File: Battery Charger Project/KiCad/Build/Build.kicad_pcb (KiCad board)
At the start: 2 copper layers, 135 x 107 mm, 63 parts, among them J1 726386-2, J10 726386-2, J11 726386-2, J2 726386-2, J3 726386-2, J4 Screw_Terminal_01x02, J5 726386-2, J6 726386-2, J7 726386-2, J8 Screw_Terminal_01x05, J9 726386-2, T1 Transformer_SP_1S, U1 LAUNCHXL-F28379D, U2 LNK6773K-TL, U3 MCS1801GS-25-P, U4 L4941BV

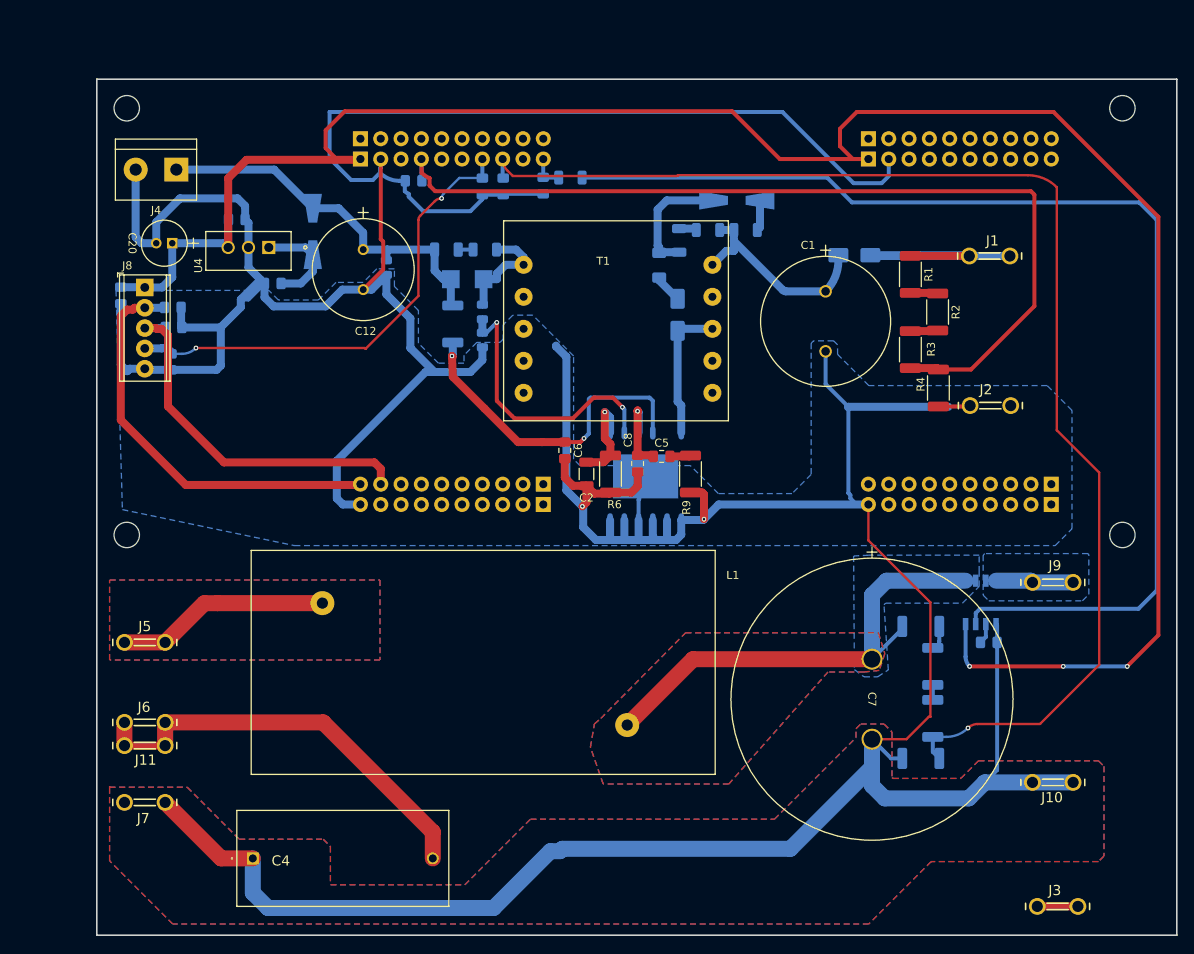
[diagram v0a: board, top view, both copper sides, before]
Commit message: More updates on PCB design
I forgot to push my changes for the last week, but I layed out the components and began routing traces and copper pours.
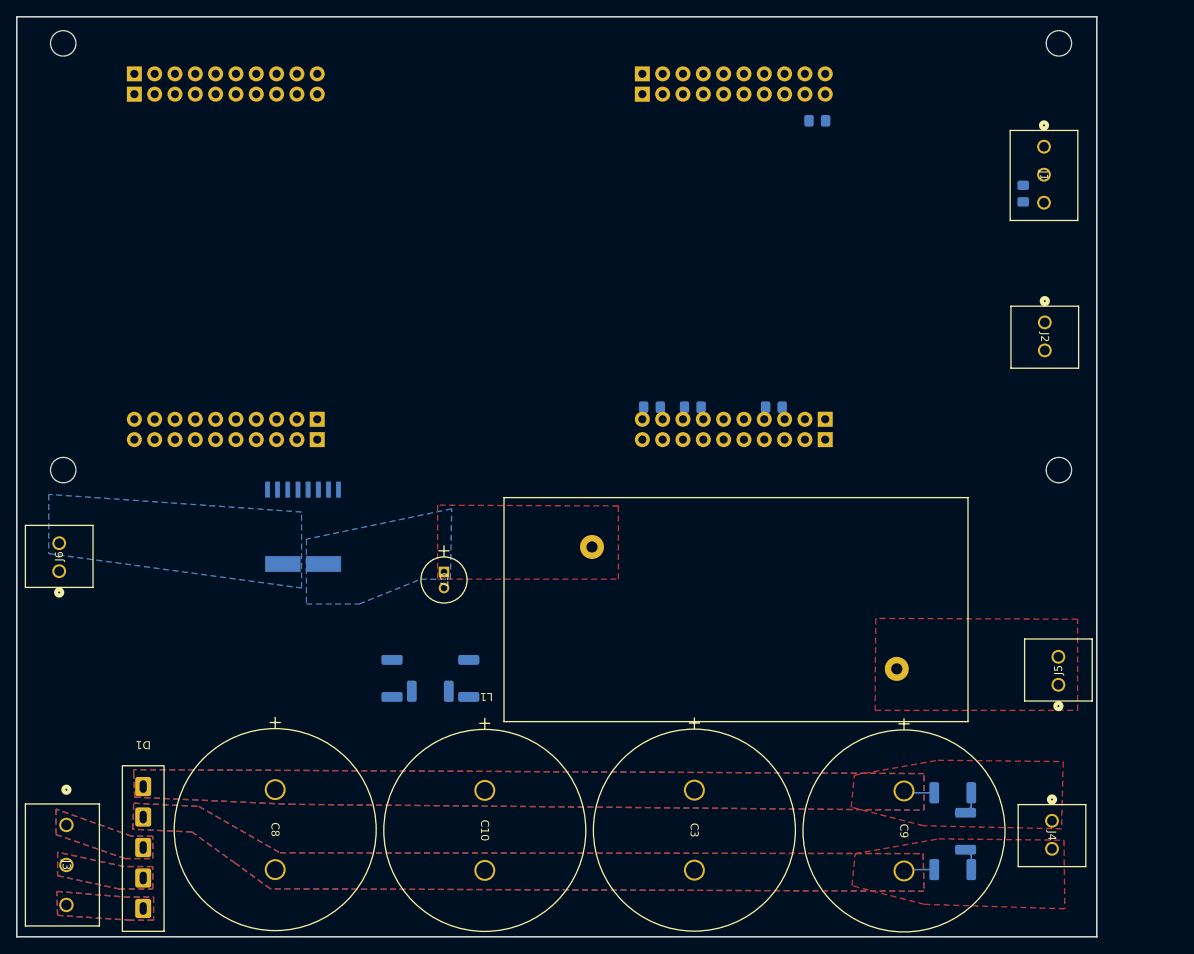
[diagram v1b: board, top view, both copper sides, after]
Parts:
- removed C11, C13, C14, C15, C16, C18, C19: C_Small, Capacitor_SMD:C_0805_2012Metric_Pad1.18x1.45mm_HandSolder
- removed C12: UHE1E102MHD6TO, footprints_C10:CAP_UAQ_12P5X20_NCH
- removed C17, C21: 0.1uF, Capacitor_SMD:C_0805_2012Metric_Pad1.18x1.45mm_HandSolder
- removed C20: ~, footprints_C20:CAP_WCAP-ATG5_05.0X11.0_WRE
- removed D2, D5: D_Zener, Diode_SMD:D_SMA-SMB_Universal_Handsoldering
- removed D3: US1M, Diode_SMD:D_SMA
- removed D4: STPS2H100U, footprints_SCHOTTKYDIODE:SMB_STM
- removed J10, J7, J9: 726386-2, KiCad:726386-2
- removed J11: 726386-2, Library:726386-2
- removed J8: Screw_Terminal_01x05, TerminalBlock_Phoenix:TerminalBlock_Phoenix_MPT-0,5-5-2.54_1x05_P2.54mm_Horizontal
- removed R10, R14, R15, R16, R17, R9: R_Small_US, Resistor_SMD:R_2010_5025Metric
- removed R11, R12, R19: R_Small_US, Resistor_SMD:R_0805_2012Metric
- removed R13: R_Small_US, Resistor_SMD:R_0805_2012Metric_Pad1.20x1.40mm_HandSolder
- removed R18, R20, R7: R_Small_US, Resistor_SMD:R_1206_3216Metric
- removed R8: R_Small_US, Resistor_SMD:R_1206_3216Metric_Pad1.30x1.75mm_HandSolder
- removed T1: Transformer_SP_1S, Library:Transformer_cust_v1
- removed U3: MCS1801GS-25-P, KiCadCS:SOIC127P600X175-8N
- removed U4: L4941BV, L4941BV:TO-220_STM
- C1: value UVR2G220MHD -> C_Small; footprint footprints_C1:CAP_UAQ_16X25_NCH -> Capacitor_SMD:C_0805_2012Metric_Pad1.18x1.45mm_HandSolder; moved to B.Cu
- C10, C3: value C_Small -> ~; footprint Capacitor_SMD:C_1206_3216Metric -> LGW2D561MELA30:CAP_A30_NCH; moved to F.Cu
- C2: footprint Capacitor_SMD:C_1206_3216Metric -> Capacitor_SMD:C_0805_2012Metric_Pad1.18x1.45mm_HandSolder; moved to B.Cu
- C4: value B32673P6225K000 -> C_Small; footprint KiCad_B326:B32673P__26.5_x_12_ -> Capacitor_SMD:C_0805_2012Metric_Pad1.18x1.45mm_HandSolder; moved to B.Cu
- C5, C6: moved to B.Cu
- C7: footprint footprints:CAP_C45_NCH -> EEU-FR1H100:CAP_PAN_5X11_PAN
- C8: value C_Small -> ~; footprint Capacitor_SMD:C_0805_2012Metric_Pad1.18x1.45mm_HandSolder -> LGW2D561MELA30:CAP_A30_NCH
- C9: value C_Small -> ~; footprint Capacitor_SMD:C_0805_2012Metric_Pad1.18x1.45mm_HandSolder -> LGW2D561MELA30:CAP_A30_NCH; moved to F.Cu
- D1: value US1M -> DNA40U2200GU; footprint Diode_SMD:D_SMA -> DPF30U200FC:DPF30U200FC; moved to F.Cu
- J1: value 726386-2 -> Screw_Terminal_01x03; footprint KiCad:726386-2 -> 284391-3:CONN3_284391-3_TEC
- J2: value 726386-2 -> Screw_Terminal_01x02; footprint KiCad:726386-2 -> 284391-2:CONN2_284391-2_TEC
- J3: value 726386-2 -> Screw_Terminal_01x03; footprint KiCad:726386-2 -> 277-1578-ND:CONN_1935174_PXC
- J4: value Screw_Terminal_01x02 -> 726386-2; footprint TerminalBlock:TerminalBlock_bornier-2_P5.08mm -> 284391-2:CONN2_284391-2_TEC
- J5, J6: footprint KiCad:726386-2 -> 284391-2:CONN2_284391-2_TEC
- L1: footprint Library:inductor_customized_v1 -> LC200-0185:LC200-0185
- R1: value R_US -> 300K; moved to B.Cu
- R2: value R_US -> 6490; moved to B.Cu
- R3: value R_US -> 36; moved to B.Cu
- R4: value R_US -> 5K; moved to B.Cu
- R5: value R_Small_US -> 680; footprint Resistor_SMD:R_1206_3216Metric -> Resistor_SMD:R_2010_5025Metric
- R6: value R_Small_US -> 680; moved to B.Cu
- U1: footprint Library:MOD_LAUNCHXL-F28379D_v2 -> LAUNCHXL-F28379D:LAUNCHXL-F28379D
- U2: value LNK6773K-TL -> TMCS1133C3A; footprint KiCad2:LNK6773KTL -> TMCS1133C5AQDVGR:TMCS1133C5AQDVGR
- moved J4 136.4 mm to (213.1, 131.4), turned to -90 degrees
- moved J3 124.3 mm to (89.9, 131.9), turned to -90 degrees
- moved D1 115.8 mm to (99.5, 134.9), turned to 180 degrees
- moved J5 114.3 mm to (213.9, 114.4), turned to 90 degrees
- moved C9 109.6 mm to (194.6, 127.7), turned to -90 degrees
- moved C4 86.2 mm to (178.3, 79.7)
- moved R5 71.4 mm to (130.6, 113.6), turned to 90 degrees
- moved R4 69.0 mm to (140.2, 113.6)
- moved C3 68.7 mm to (168.4, 127.6)
- moved U1 67.9 mm to (216.5, 31.7), turned to 180 degrees
- moved C10 67.8 mm to (142.2, 127.6), turned to -90 degrees
- moved R3 65.2 mm to (200.7, 137.5), turned to 180 degrees
- moved R1 65.0 mm to (200.7, 127.9), turned to 0 degrees
- moved R2 65.0 mm to (202.3, 132.7)
- moved C2 64.9 mm to (209.5, 53.0), turned to 90 degrees
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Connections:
- C1 pad 1: Net-(D1-K) -> PWMA
- C10 pad 1: Net-(C10-Pad1) -> VHV
- C10 pad 2: 12V -> GND
- C2 pad 1: Net-(U2-PD) -> 5V
- C3 pad 1: Net-(C3-Pad1) -> VHV
- C3 pad 2: Net-(D2-K) -> GND
- C4 pad 1: GND -> VHV_S
- C4 pad 2: Net-(C4-Pad2) -> GND
- C5 pad 1: Net-(U2-CP) -> Vo_S
- C5 pad 2: Net-(C5-Pad2) -> GND
- C6 pad 1: Net-(U2-BP) -> Io_S
- C7 pad 1: Net-(U3-IP+_1) -> Net-(U2-IN+)
- C8 pad 1: Net-(U2-CP) -> VHV
- C9 pad 1: PWMA -> VHV
- D1 pad 1: Net-(D1-K) -> VHV
- D1 pad 2: VHV -> GND
- J1 pad 1: VHV -> GND
- J1 pad 2: VHV -> PWMA
- J2 pad 1: GND -> 5V
- J3 pad 1: unconnected-(J3-Pad1) -> /A
- J3 pad 2: unconnected-(J3-Pad1) -> /B
- J4 pad 1: 12V -> VHV
- J6 pad 1: Net-(C4-Pad2) -> GND
- J6 pad 2: Net-(C4-Pad2) -> Vo
- L1 pad 2: Net-(U3-IP+_1) -> Net-(U2-IN+)
- R1 pad 2: Net-(R1-Pad2) -> VHV_S
- R2 pad 1: Net-(R1-Pad2) -> VHV_S
- R3 pad 2: VHV1 -> GND
- R4 pad 1: VHV1 -> Net-(U2-IN+)
- R4 pad 2: GND -> Vo_S
- R5 pad 1: Net-(D1-K) -> Net-(R5-Pad1)
- R5 pad 2: Net-(D2-A) -> GND
- R6 pad 1: Net-(U2-PD) -> Vo_S
- R6 pad 2: GND -> Net-(R5-Pad1)
- U1 pad J3_10: Net-(U1C-ADCINA0/ANALOGIN(DACA)) -> Io_S
- U1 pad J3_4: VHV1 -> VHV_S
- U1 pad J3_7: Board Temp -> unconnected-(U1C-ADCINC2/ANALOGIN-PadJ3_7)
- U1 pad J3_8: Vo -> Vo_S
- U1 pad J4_9: PWMB -> unconnected-(U1D-GPIO1/PWMOUT1B-PadJ4_9)
- U2 pad 1: Net-(U2-PD) -> Net-(U2-IN+)
- U2 pad 10: GND -> (no net)
- U2 pad 2: Net-(U2-FB) -> Vo
- U2 pad 3: Net-(U2-CP) -> GND
- U2 pad 4: Net-(U2-BP) -> (no net)
- U2 pad 6: Net-(D3-A) -> Io_S
- U2 pad 7: GND -> (no net)
- U2 pad 8: GND -> (no net)
- U2 pad 9: GND -> +5V
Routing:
- net GND: track 624.9 -> 3.86 mm, vias 2 -> 0
- net 5V: track 260.0 -> 0.00 mm, vias 3 -> 0
- net Vo: track 162.5 -> 0.00 mm, vias 1 -> 0
- net Ibatt: track 145.5 -> 0.00 mm
- net VHV1: track 115.5 -> 0.00 mm
- net Net-(U3-IP+_1): track 60.1 -> 0.00 mm
- net Board Temp: track 59.9 -> 0.00 mm, vias 2 -> 0
- net Net-(C4-Pad2): track 53.3 -> 0.00 mm
- net PWMA: track 52.2 -> 0.00 mm
- net 12V: track 47.9 -> 0.00 mm
- net PWMB: track 46.6 -> 0.00 mm
- net Net-(U2-BP): track 41.8 -> 0.00 mm, vias 2 -> 0
- net Net-(U2-FB): track 35.3 -> 0.00 mm, vias 2 -> 0
- net VHV: track 37.2 -> 3.88 mm
- net Net-(J5-Pad1): track 26.8 -> 0.00 mm
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- added copper zone on B.Cu, net /A
- added copper zone on F.Cu, net /A
- added copper zone on B.Cu, net /B
- added copper zone on F.Cu, net /B
- added copper zone on B.Cu, net /C
- added copper zone on F.Cu, net /C
- added copper zone on B.Cu, net Net-(U2-IN+)
- added copper zone on F.Cu, net Net-(U2-IN+)
- added copper zone on B.Cu, net VHV
- added copper zone on F.Cu, net VHV
- added copper zone on B.Cu, net Vo
- removed copper zone on B.Cu, net IP-
- removed copper zone on B.Cu, net Net-(J5-Pad1)
- removed copper zone on B.Cu, net Net-(U3-IP+_1)
- removed copper zone on F.Cu, net Net-(U3-IP+_1)
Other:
- board size 135 x 107 mm -> 135 x 115 mm
